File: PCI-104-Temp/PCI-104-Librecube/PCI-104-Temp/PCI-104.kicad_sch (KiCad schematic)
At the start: 6 parts, among them J3 Conn_02x26_Row_Letter_First, J4 Conn_02x26_Row_Letter_First

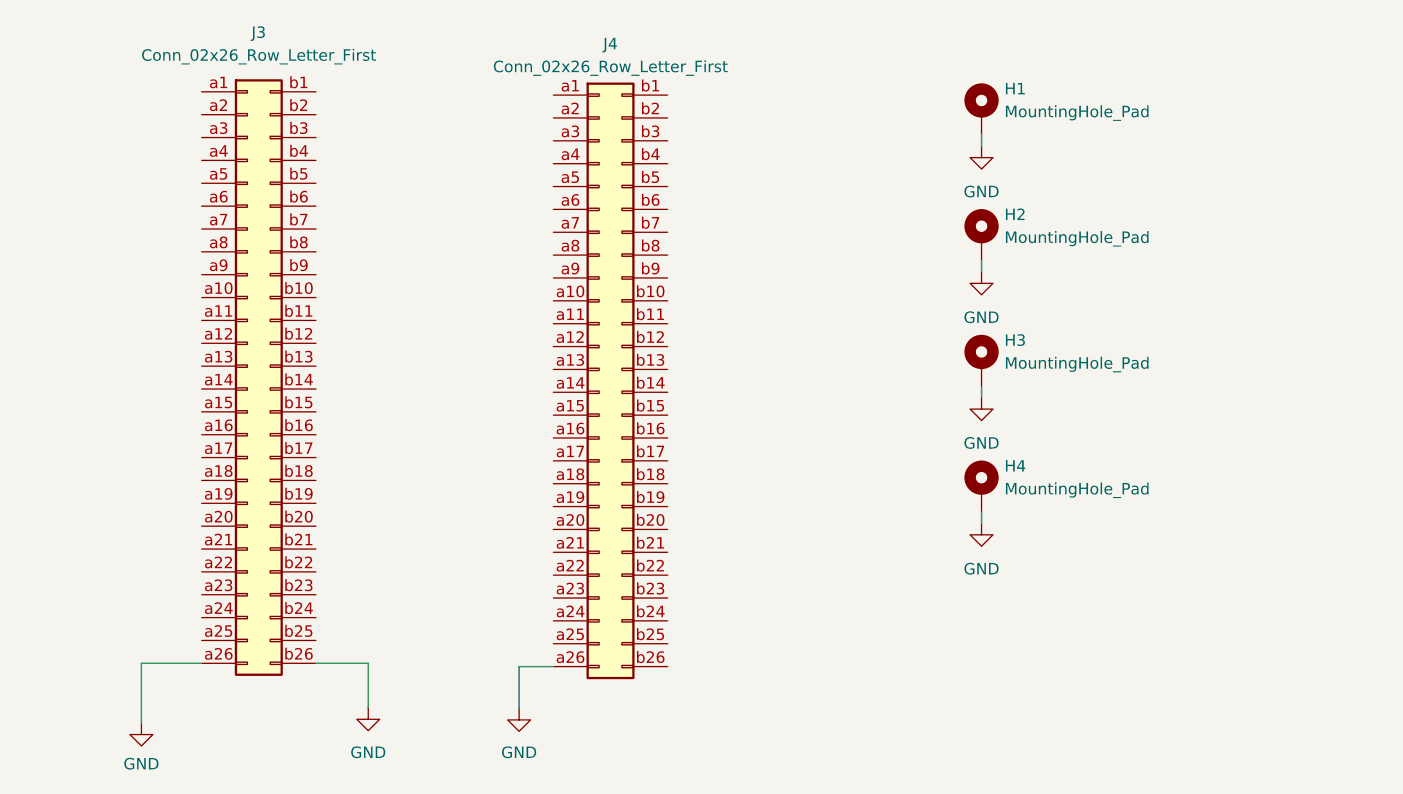
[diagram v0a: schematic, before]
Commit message: EPS PCB Ready for Order
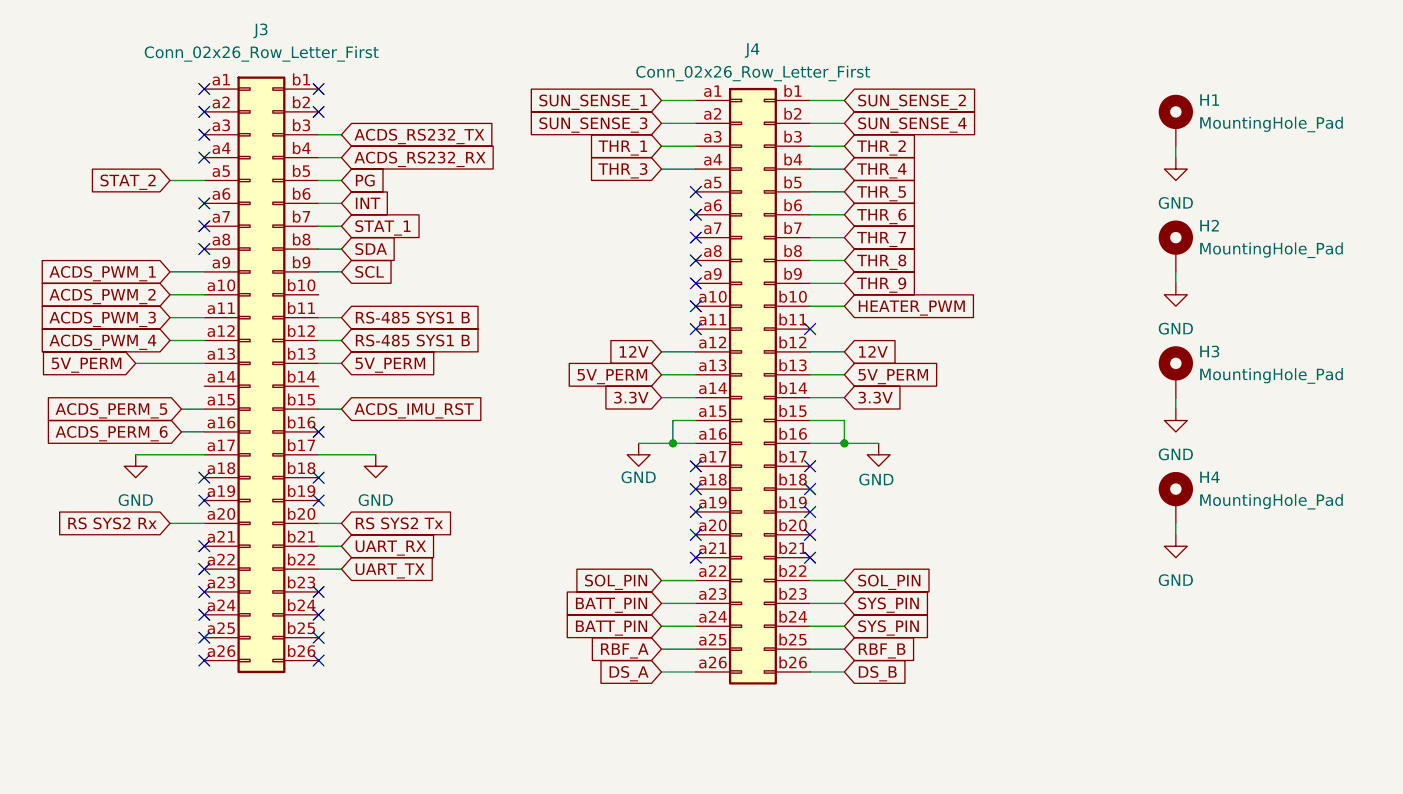
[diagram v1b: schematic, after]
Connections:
- net GND: now also J3.a17 (Pin_a17), J3.b17 (Pin_b17), J4.a15 (Pin_a15), J4.a16 (Pin_a16), J4.b15 (Pin_b15), J4.b16 (Pin_b16); no longer J3.a26 (Pin_a26), J3.b26 (Pin_b26), J4.a26 (Pin_a26)
- net ACDS_PWM_2: now reaches J3.a10 (Pin_a10)
- net ACDS_PWM_3: now reaches J3.a11 (Pin_a11)
- net ACDS_PWM_4: now reaches J3.a12 (Pin_a12)
- net 5V_PERM: now reaches J3.a13 (Pin_a13)
- net 5V_PERM: now also J3.b13 (Pin_b13), J4.a13 (Pin_a13), J4.b13 (Pin_b13)
- net ACDS_PERM_5: now reaches J3.a15 (Pin_a15)
- net ACDS_PERM_6: now reaches J3.a16 (Pin_a16)
- net RS SYS2 Rx: now reaches J3.a20 (Pin_a20)
- net STAT_2: now reaches J3.a5 (Pin_a5)
- net ACDS_PWM_1: now reaches J3.a9 (Pin_a9)
- net RS-485 SYS1 B: now reaches J3.b11 (Pin_b11)
- net RS-485 SYS1 B: now also J3.b12 (Pin_b12)
- net ACDS_IMU_RST: now reaches J3.b15 (Pin_b15)
- net RS SYS2 Tx: now reaches J3.b20 (Pin_b20)
- net UART_RX: now reaches J3.b21 (Pin_b21)
- net UART_TX: now reaches J3.b22 (Pin_b22)
- net ACDS_RS232_TX: now reaches J3.b3 (Pin_b3)
- net ACDS_RS232_RX: now reaches J3.b4 (Pin_b4)
- net PG: now reaches J3.b5 (Pin_b5)
- net INT: now reaches J3.b6 (Pin_b6)
- net STAT_1: now reaches J3.b7 (Pin_b7)
- net SDA: now reaches J3.b8 (Pin_b8)
- net SCL: now reaches J3.b9 (Pin_b9)
- net SUN_SENSE_1: now reaches J4.a1 (Pin_a1)
- net 12V: now reaches J4.a12 (Pin_a12)
- net 12V: now also J4.b12 (Pin_b12)
- net 3.3V: now reaches J4.a14 (Pin_a14)
- net 3.3V: now also J4.b14 (Pin_b14)
- net SUN_SENSE_3: now reaches J4.a2 (Pin_a2)
- net SOL_PIN: now reaches J4.a22 (Pin_a22)
- net SOL_PIN: now also J4.b22 (Pin_b22)
- net BATT_PIN: now reaches J4.a23 (Pin_a23)
- net BATT_PIN: now also J4.a24 (Pin_a24)
- net RBF_A: now reaches J4.a25 (Pin_a25)
- net THR_1: now reaches J4.a3 (Pin_a3)
- net THR_3: now reaches J4.a4 (Pin_a4)
- net SUN_SENSE_2: now reaches J4.b1 (Pin_b1)
- net HEATER_PWM: now reaches J4.b10 (Pin_b10)
- net SUN_SENSE_4: now reaches J4.b2 (Pin_b2)
- net SYS_PIN: now reaches J4.b23 (Pin_b23)
- net SYS_PIN: now also J4.b24 (Pin_b24)
- net RBF_B: now reaches J4.b25 (Pin_b25)
- net DS_B: now reaches J4.b26 (Pin_b26)
- net THR_2: now reaches J4.b3 (Pin_b3)
- net THR_4: now reaches J4.b4 (Pin_b4)
- net THR_5: now reaches J4.b5 (Pin_b5)
- net THR_6: now reaches J4.b6 (Pin_b6)
- net THR_7: now reaches J4.b7 (Pin_b7)
- net THR_8: now reaches J4.b8 (Pin_b8)
- net THR_9: now reaches J4.b9 (Pin_b9)
- new net DS_A: J4.a26 (Pin_a26)
- no-connect marks 0 -> 42
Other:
- moved on the sheet: H1, H2, H3, H4, J4

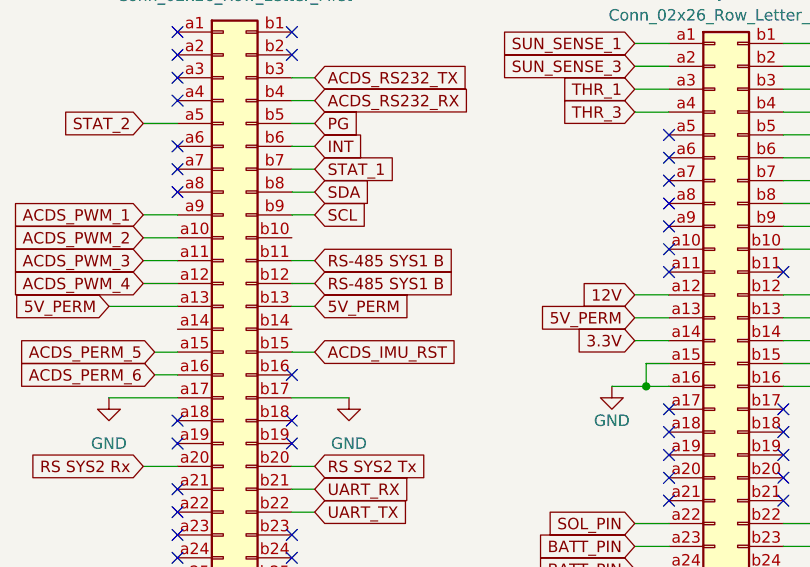
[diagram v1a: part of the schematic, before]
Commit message: Small PC104 Template Fix
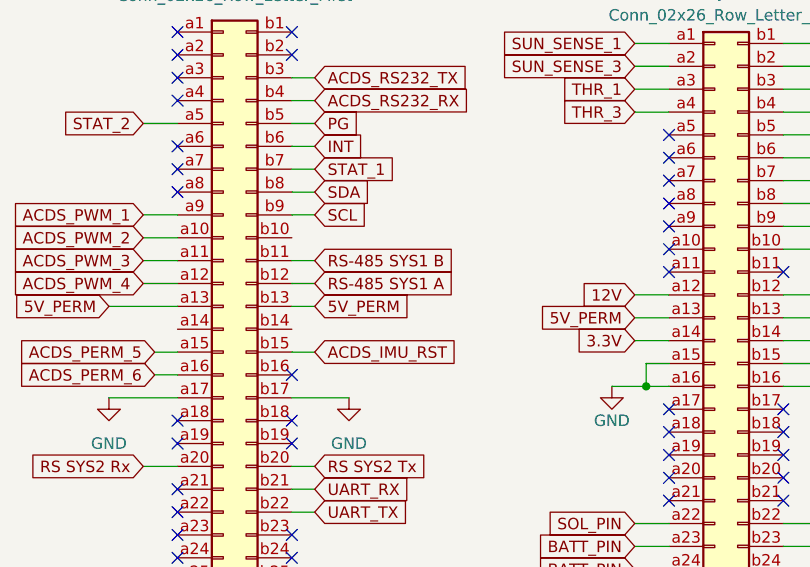
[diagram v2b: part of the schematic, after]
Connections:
- net RS-485 SYS1 B: no longer J3.b12 (Pin_b12)
- new net RS-485 SYS1 A: J3.b12 (Pin_b12)
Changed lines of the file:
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@@
 		)
 	)
-	(global_label "RS-485 SYS1 B"
+	(global_label "RS-485 SYS1 A"
 		(shape input)
 		(at 182.88 82.55 0)
@@
 		)
 		(property "Intersheetrefs" "${INTERSHEET_REFS}"
-			(at 201.4679 82.55 0)
+			(at 201.2865 82.55 0)
 			(hide yes)
 			(show_name no)
